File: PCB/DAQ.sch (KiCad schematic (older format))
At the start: 62 parts, among them IC1 MAX743CWE+, J1 Arduino_Mega_Header, J2 Conn_01x07, J3 Conn_01x08, J4 Conn_01x08, J5 Conn_02x18_Counter_Clockwise, J6 Conn_01x10, J7 Conn_01x08, J8 Conn_01x07, J9 Screw_Terminal_01x08, U1 SDshield, U10 ADG408, U2 RTC, U3 ADC, U4 NOKIA5110, U5 DAC, U6 LM358, U7 LM358, U8 LM358, U9 LM358

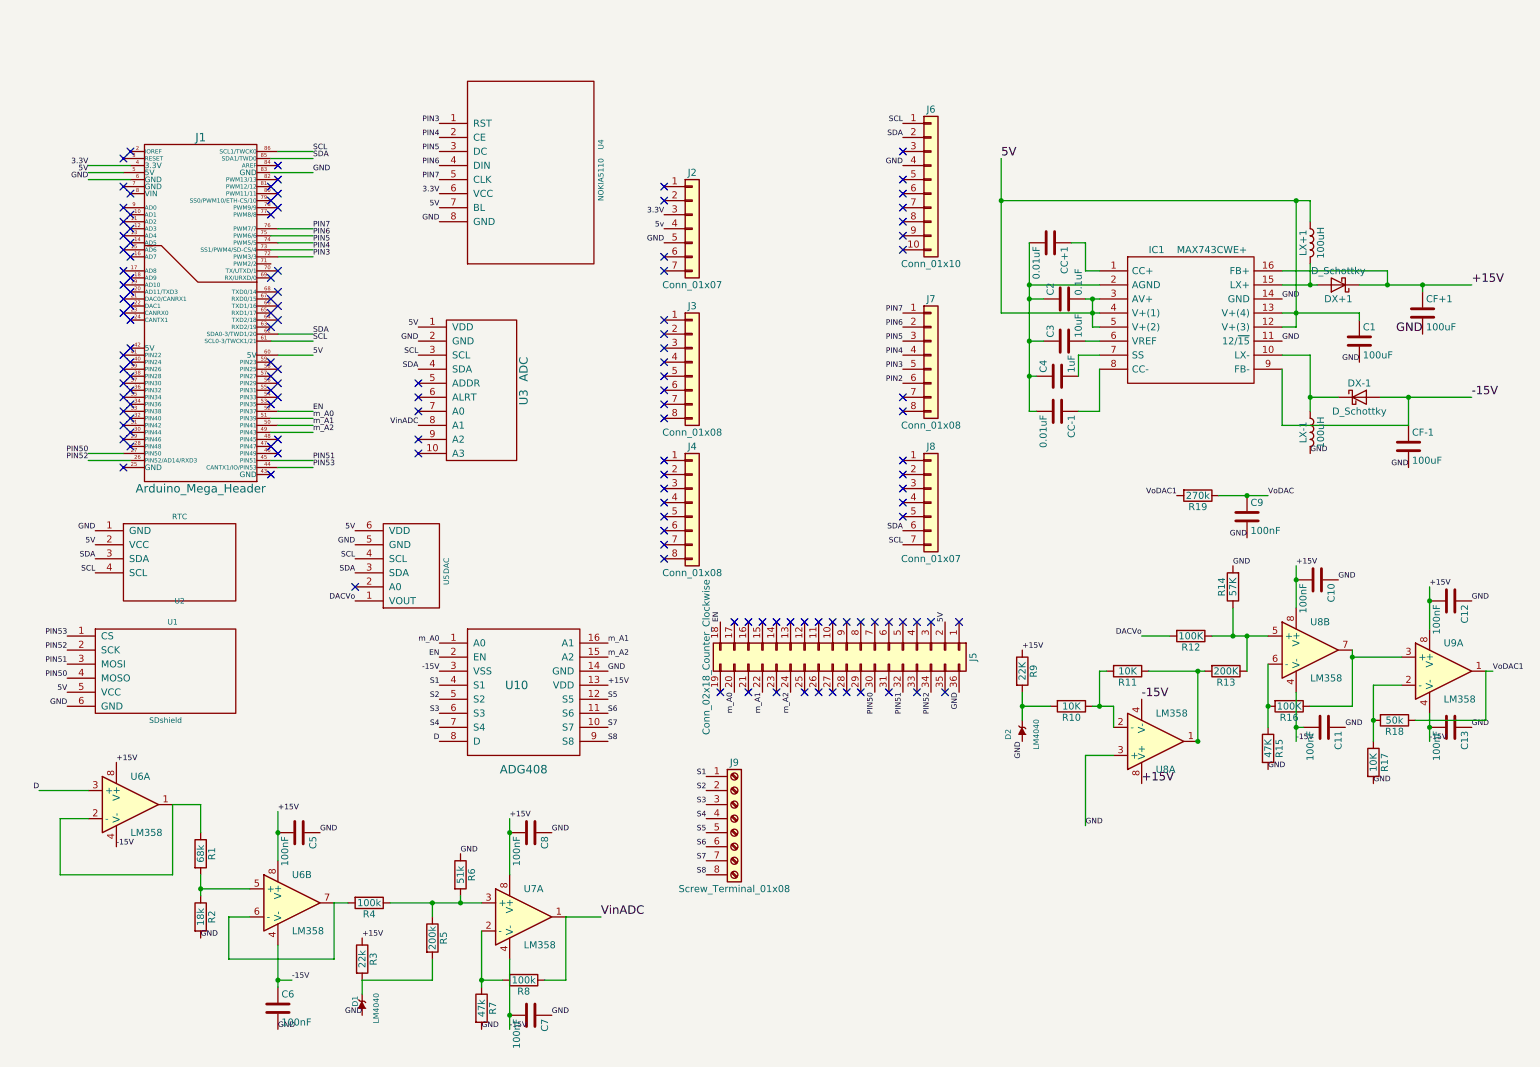
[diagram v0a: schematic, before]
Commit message: New version of PCB
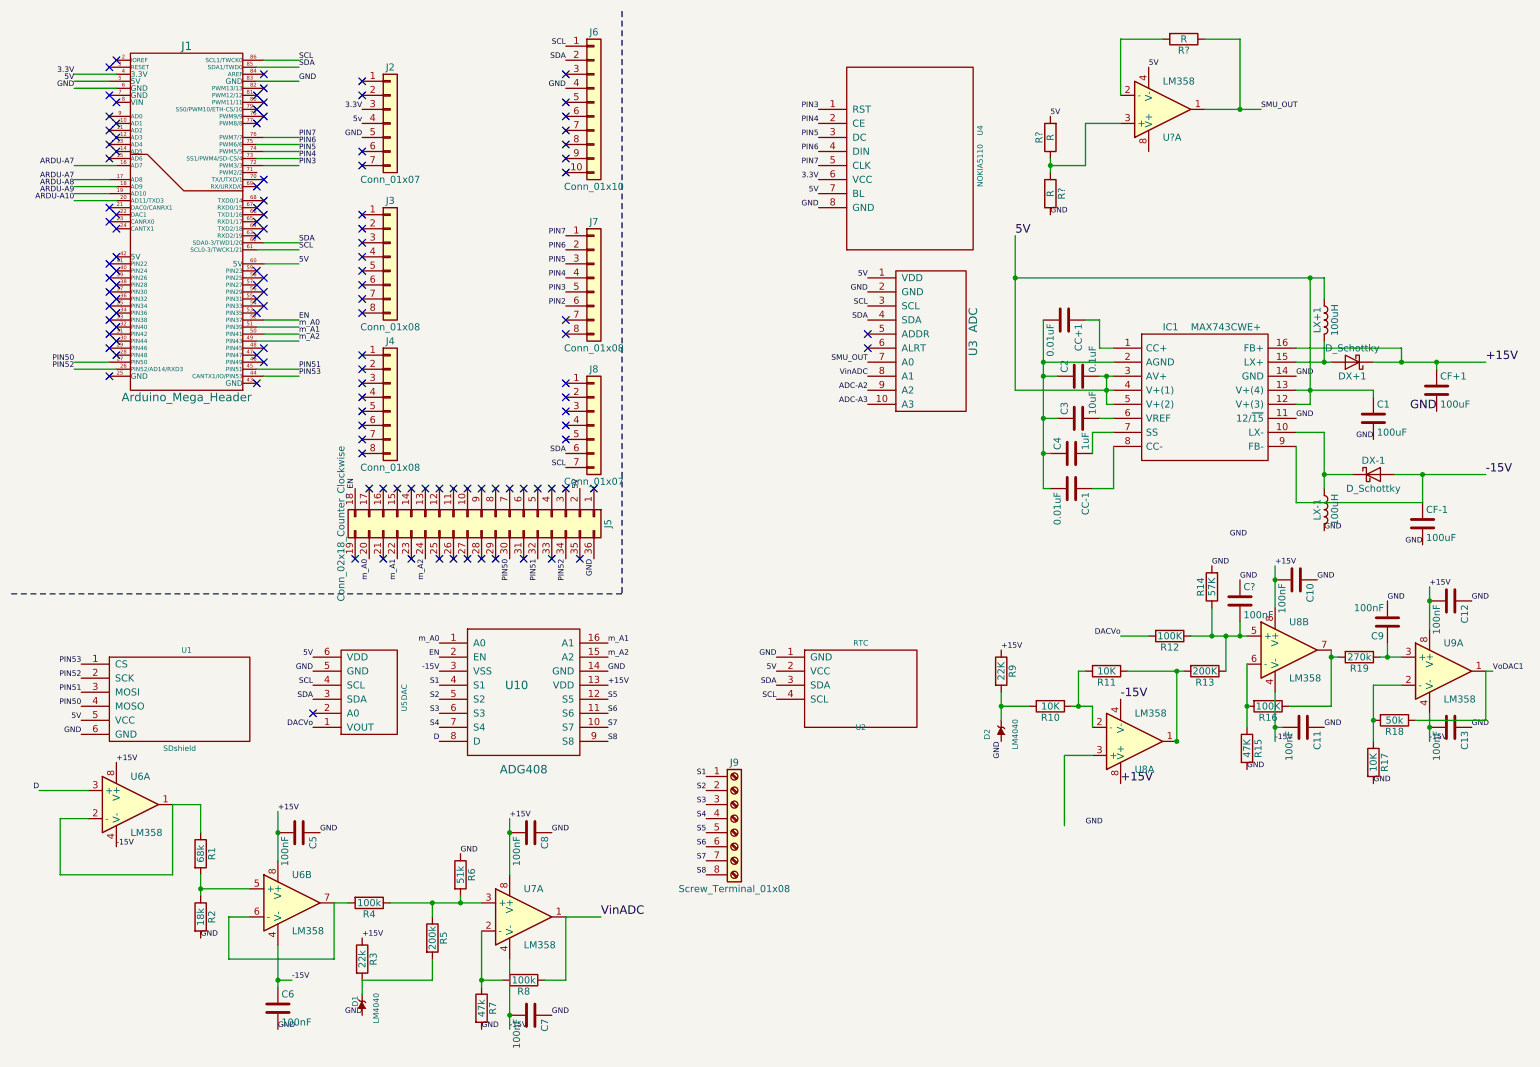
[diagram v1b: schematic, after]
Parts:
- added C?: 100nF, symbol C
- added R? (x3): R, symbol R
- added U?: LM358, symbol LM358
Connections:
- net 5V: now also R?.2, U?.4 (V-)
- net GND: now also C?.1, R?.2; no longer U8.3 (+)
- net VoDAC1: no longer R19.2
- net ARDU-A7: now reaches J1.16 (AD7)
- net ARDU-A7: now also J1.17 (AD8)
- net ARDU-A8: now reaches J1.18 (AD9)
- net ARDU-A9: now reaches J1.19 (AD10)
- net ARDU-A10: now reaches J1.20 (AD11/TXD3)
- net ADC-A3: now reaches U3.10 (A3)
- net SMU_OUT: now reaches U3.7 (A0)
- net SMU_OUT: now also R?.1, U?.1
- net ADC-A2: now reaches U3.9 (A2)
- net at R16.1, U8.7: now also R19.2; no longer U9.3 (+)
- net at R12.1, R13.1, R14.1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: now also C?.2
- net VoDAC: no longer names the net of C9.1, R19.1
- net VoDAC: now also U9.3 (+)
- new net: R?.2, U?.2 (-)
- new net: R?.1, R?.1, U?.3 (+)
- no-connect marks 129 -> 121
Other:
- moved on the sheet: C1, C10, C11, C2, C3, C4, C9, CC+1, CC-1, CF+1, CF-1, D2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
